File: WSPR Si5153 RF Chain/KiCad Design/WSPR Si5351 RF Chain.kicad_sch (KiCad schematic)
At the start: 0 parts

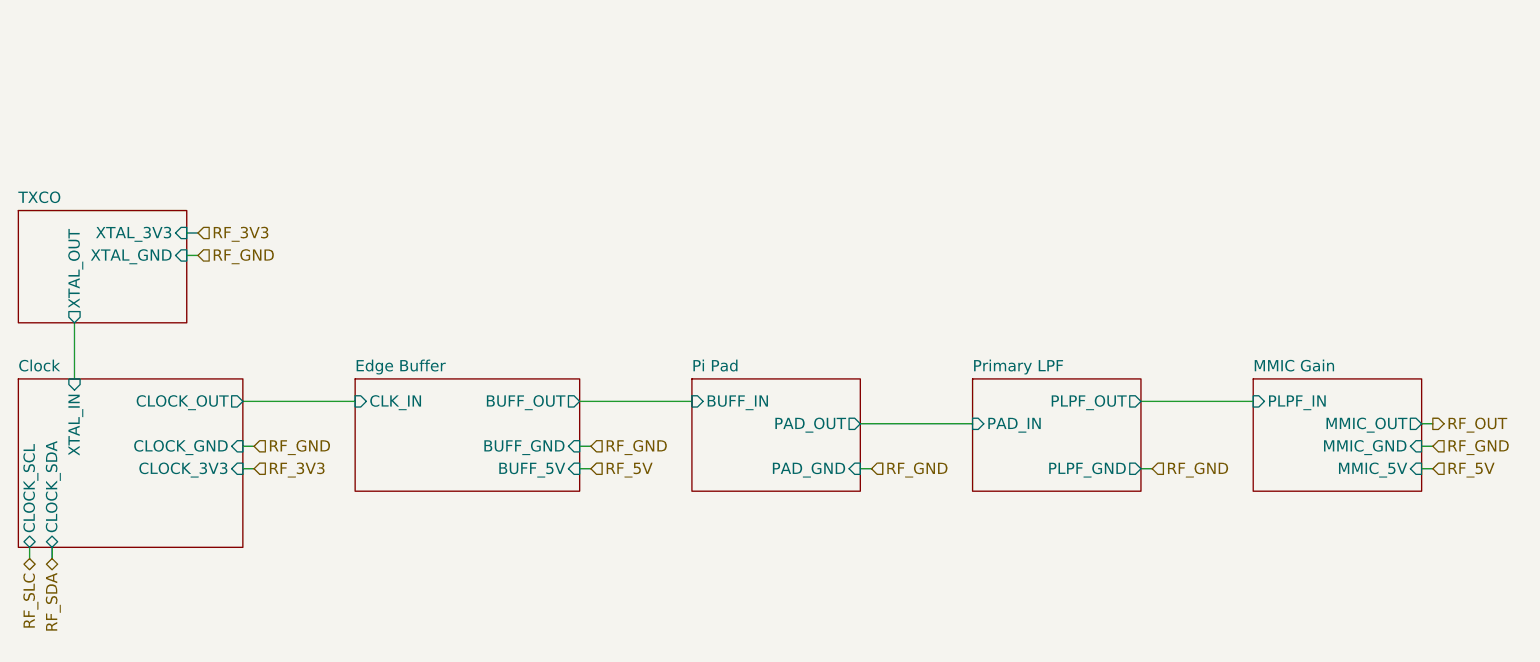
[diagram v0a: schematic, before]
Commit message: Notionally complete through PA
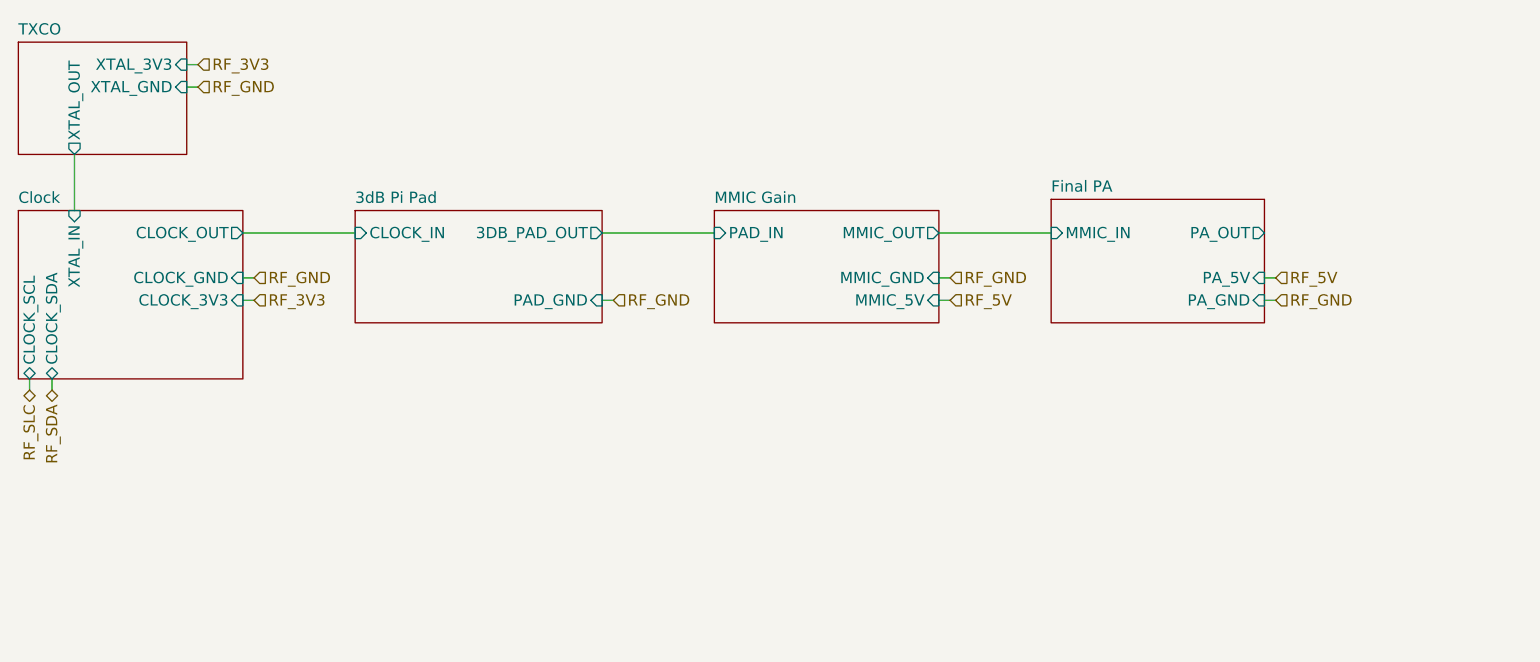
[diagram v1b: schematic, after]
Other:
- sheet Pi Pad renamed 3dB Pi Pad
- removed sheet Edge Buffer
- removed sheet Primary LPF
- added sheet Final PA (../Components/PA/KiCad Design/PA.kicad_sch)
- sheet 3dB Pi Pad: file ../../WSPR Si5153 RF Chain/Components/6dB Pi Pad/KiCad Design/6dB Pad.kicad_sch -> ../../WSPR Si5153 RF Chain/Components/3dB Pi Pad/KiCad Design/3dB Pad.kicad_sch
- sheet 3dB Pi Pad ports: added 3DB_PAD_OUT, CLOCK_IN; removed BUFF_IN, PAD_OUT
- sheet MMIC Gain ports: added PAD_IN; removed PLPF_IN
